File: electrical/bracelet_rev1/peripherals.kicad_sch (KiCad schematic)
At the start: 18 parts, among them SW2 SW_MEC_5E, U6 LSM6DS3, U7 MAX30102, U8 TXS0101DBV, U9 BMP390L

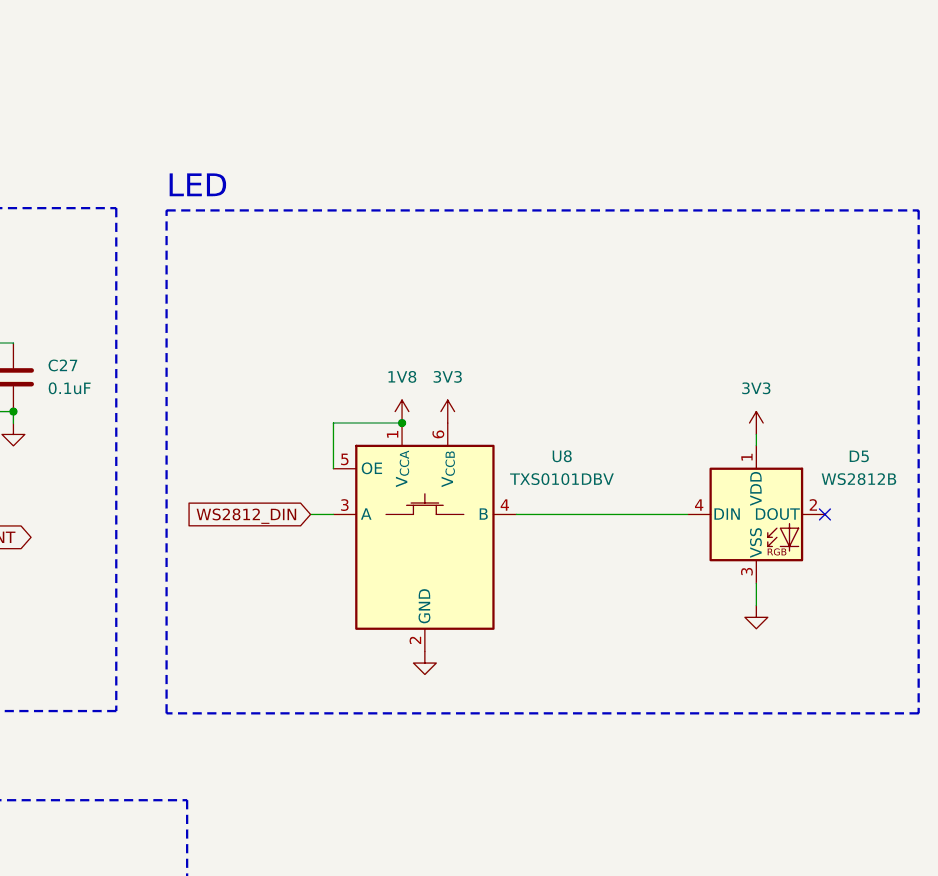
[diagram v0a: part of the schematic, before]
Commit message: Updated more things
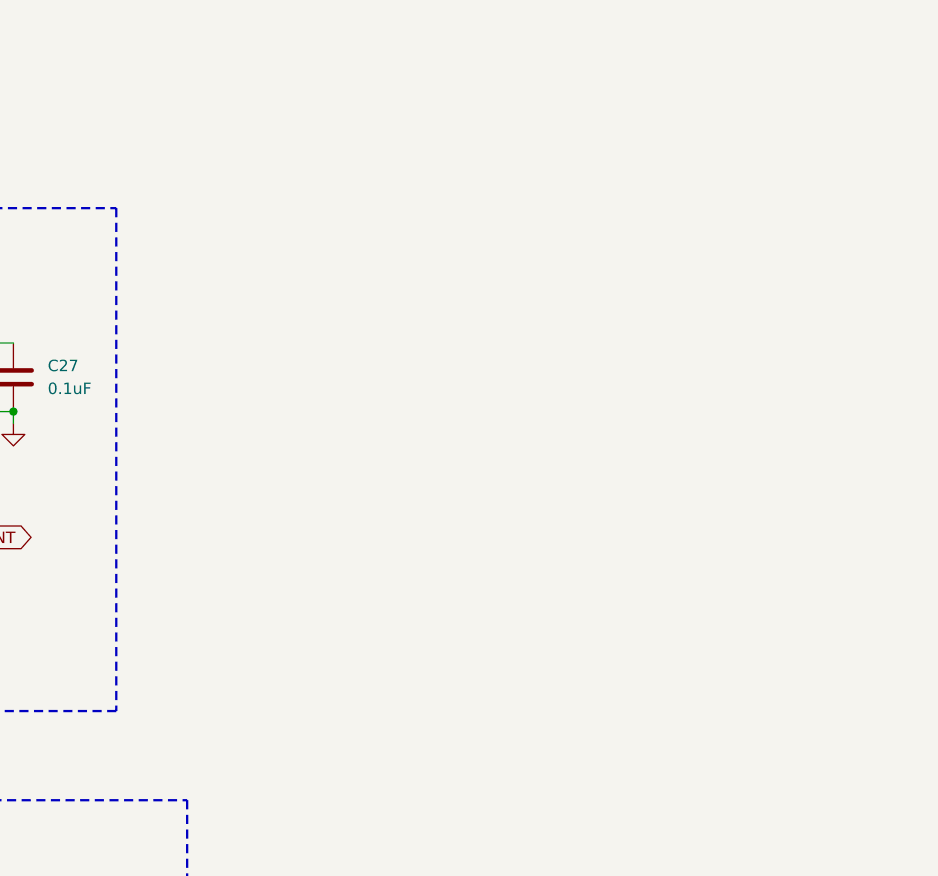
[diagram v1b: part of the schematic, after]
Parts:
- removed D5: WS2812B, LED_SMD:LED_WS2812B_PLCC4_5.0x5.0mm_P3.2mm, symbol LED:WS2812B
- removed U8: TXS0101DBV, Package_TO_SOT_SMD:SOT-23-6, symbol Logic_LevelTranslator:TXS0101DBV
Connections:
- no-connect marks 1 -> 0
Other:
- note removed: "LED"

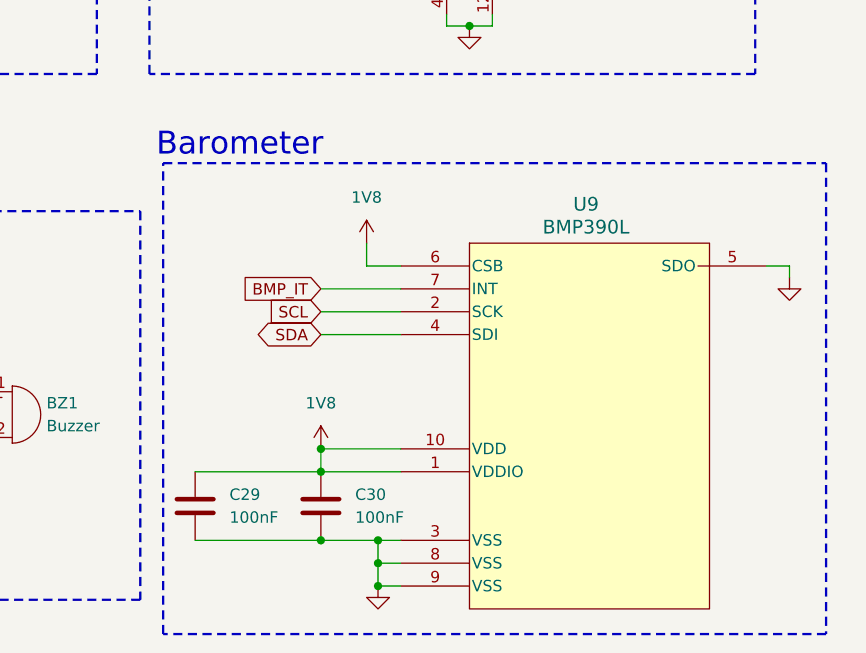
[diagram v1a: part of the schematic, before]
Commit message: More schematic stuff
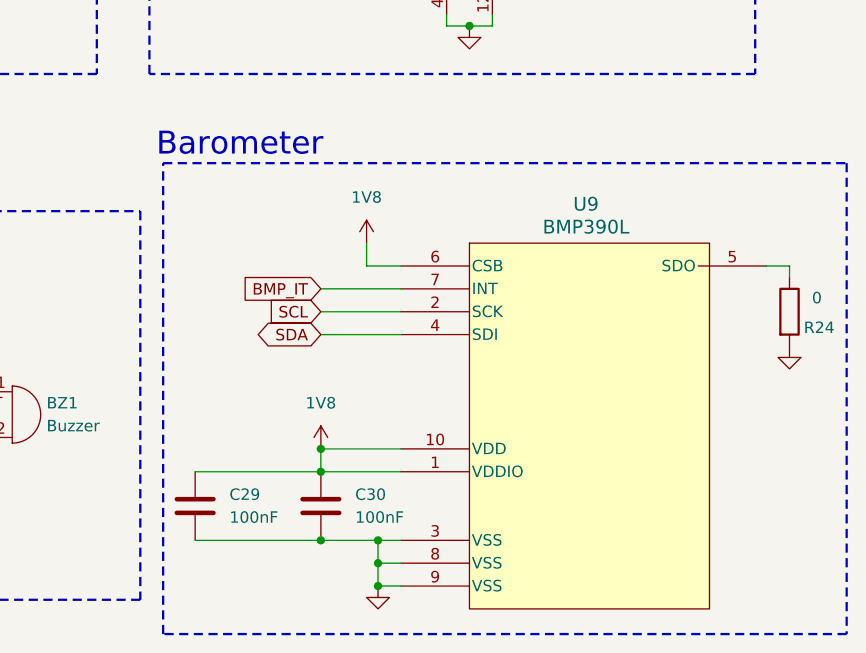
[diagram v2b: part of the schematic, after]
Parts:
- added R24: 0, Resistor_SMD:R_0201_0603Metric_Pad0.64x0.40mm_HandSolder, symbol Device:R
- C22, C23, C24, C25, C26, C27, C28, C29, C30: footprint (none) -> Capacitor_SMD:C_0603_1608Metric_Pad1.08x0.95mm_HandSolder
- R19, R20: footprint (none) -> Resistor_SMD:R_0603_1608Metric_Pad0.98x0.95mm_HandSolder
- SW2: footprint (none) -> Button_Switch_SMD:SW_MEC_5GSH9
- U9: footprint 10LGA_2X2X0p75_BOS -> (none)
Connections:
- net GND: now also R24.2; no longer U9.5 (SDO)
- new net: R24.1, U9.5 (SDO)
